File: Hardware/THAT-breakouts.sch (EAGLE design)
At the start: 27 parts, among them IC1 THAT1206, IC2 THAT1646, J1 INPUT, J2 OUTPUT, J3 CHASSIS

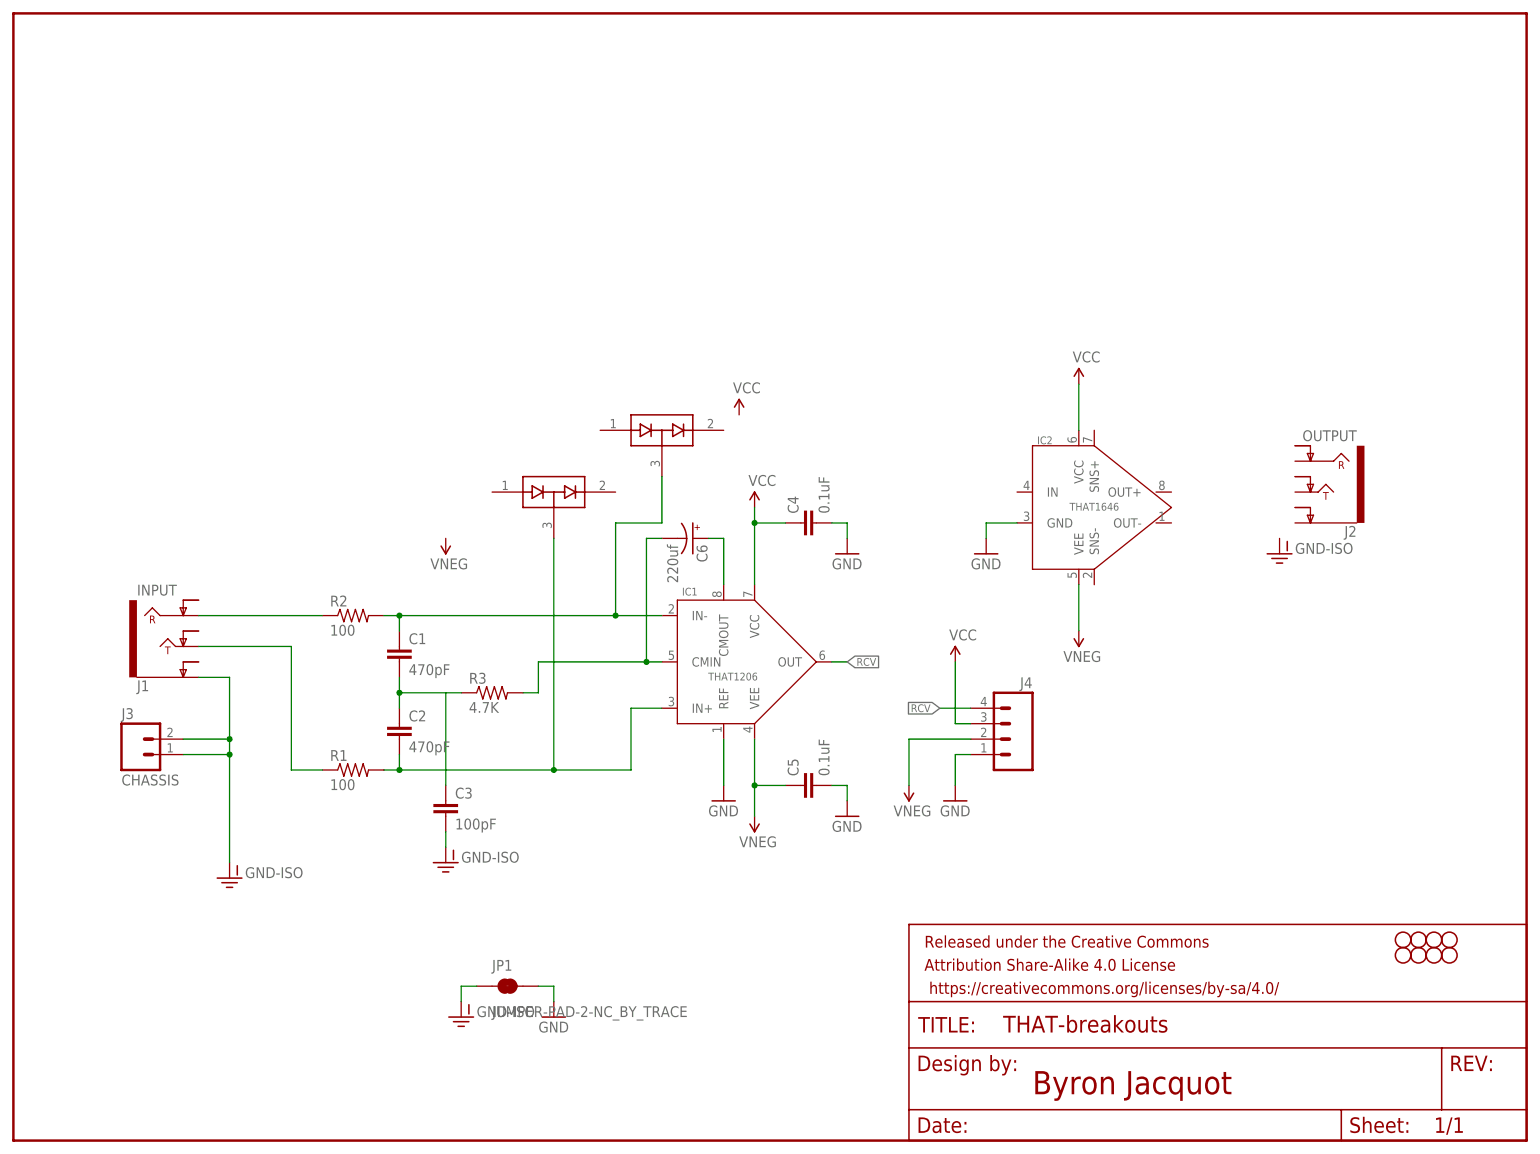
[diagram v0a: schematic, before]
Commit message: More WIP & conceptual work.
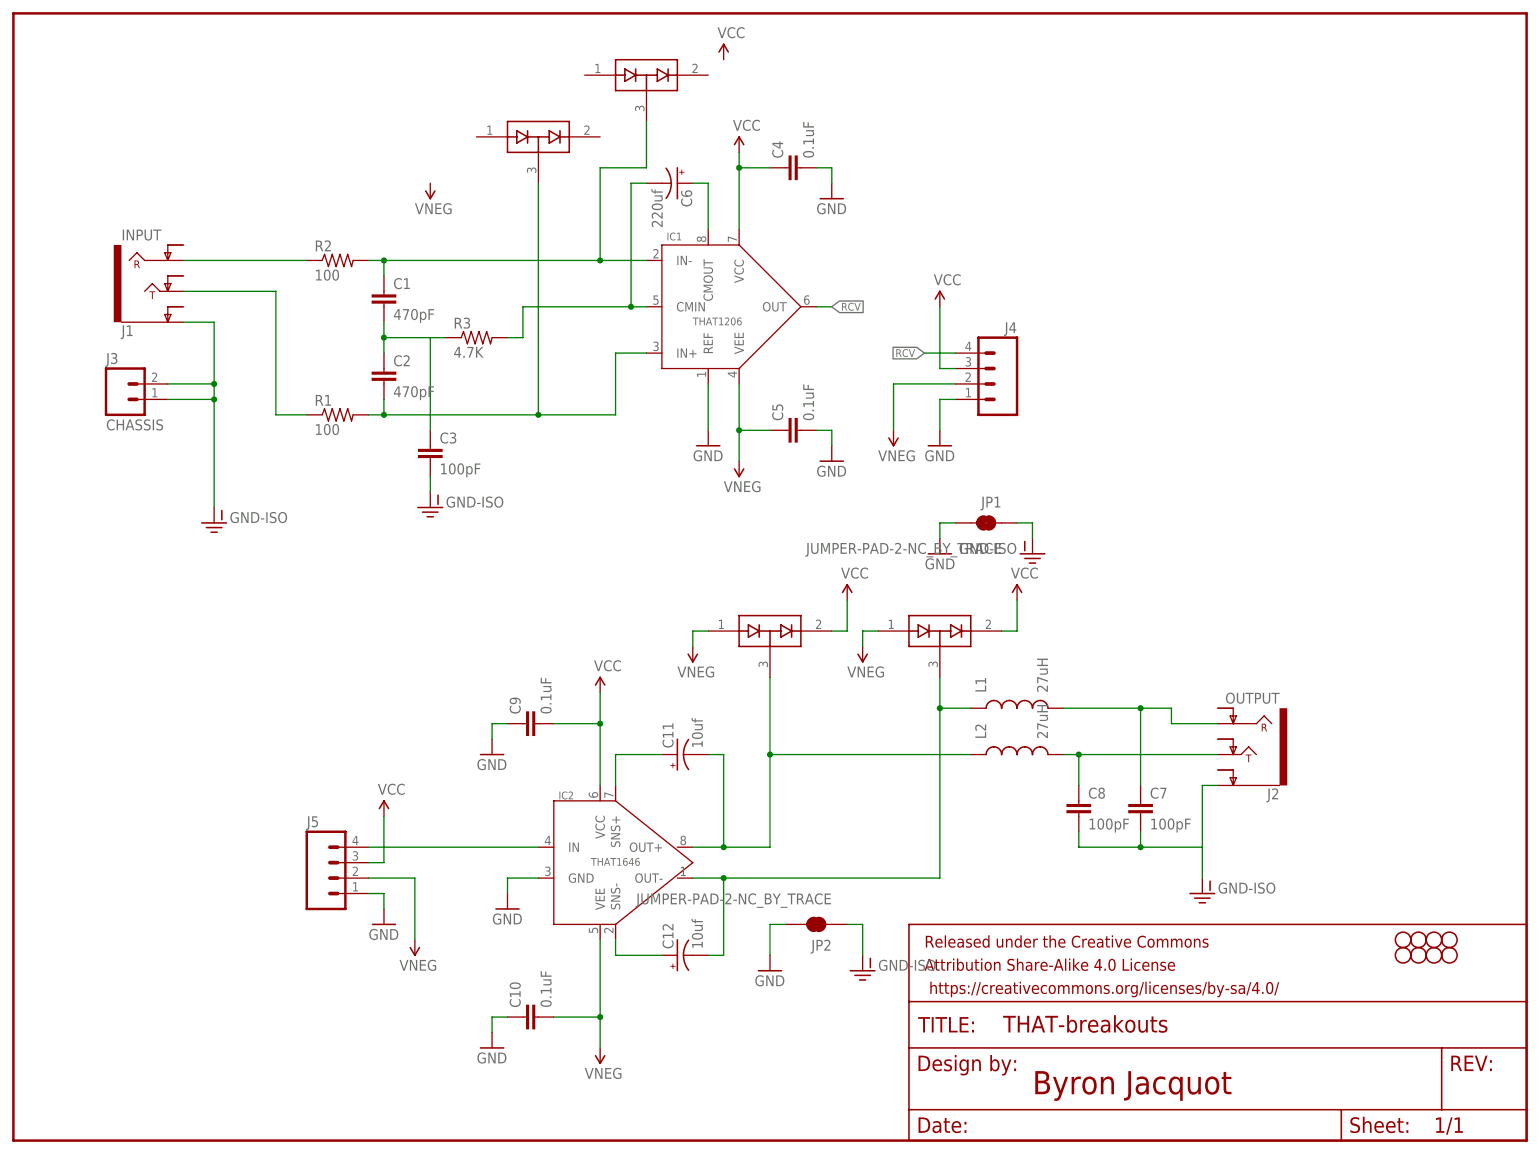
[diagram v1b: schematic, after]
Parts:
- added C10, C9: 0.1uF, SparkFun-Capacitors:0.1UF-25V-5%(0603)
- added C11, C12: 10uf, that-ics:PANA-EEE-1EA100NP
- added C7, C8: 100pF, SparkFun-Capacitors:100PF-50V-5%(0603)
- added D1, D2: (no value), SparkFun-DiscreteSemi:BAV99
- added J5: (no value), SparkFun-Connectors:M04NO_SILK_ALL_ROUND
- added JP2: JUMPER-PAD-2-NC_BY_TRACE, SparkFun-Passives:JUMPER-PAD-2-NC_BY_TRACE
- added L1, L2: 27uH, SparkFun-Passives:INDUCTOR0603
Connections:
- new net N$10: C11.-, D2.COM, IC2.OUT+, L2.1
- new net N$11: C12.-, D1.COM, IC2.OUT-, L1.1
- new net N$13: C12.+, IC2.SNS-
- new net N$14: C11.+, IC2.SNS+
- new net N$16: IC2.IN, J5.4
- new net N$8: C8.1, J2.TIP, L2.2
- new net N$9: C7.1, J2.RING, L1.2
- net GND: now also C10.1, C9.1, J5.1, JP2.2
- net GND-ISO: now also C7.2, C8.2, J2.EARTH, JP2.1
- net VCC: now also C9.2, D1.C2, D2.C2, J5.3
- net VNEG: now also C10.2, D1.A1, D2.A1, J5.2
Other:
- moved on the sheet: C1, C2, C3, C4, C5, C6, IC1, IC2, J1, J2, J3, J4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
